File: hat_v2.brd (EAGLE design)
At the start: 65 x 56.5 mm, 18 parts, among them IC1 4N35

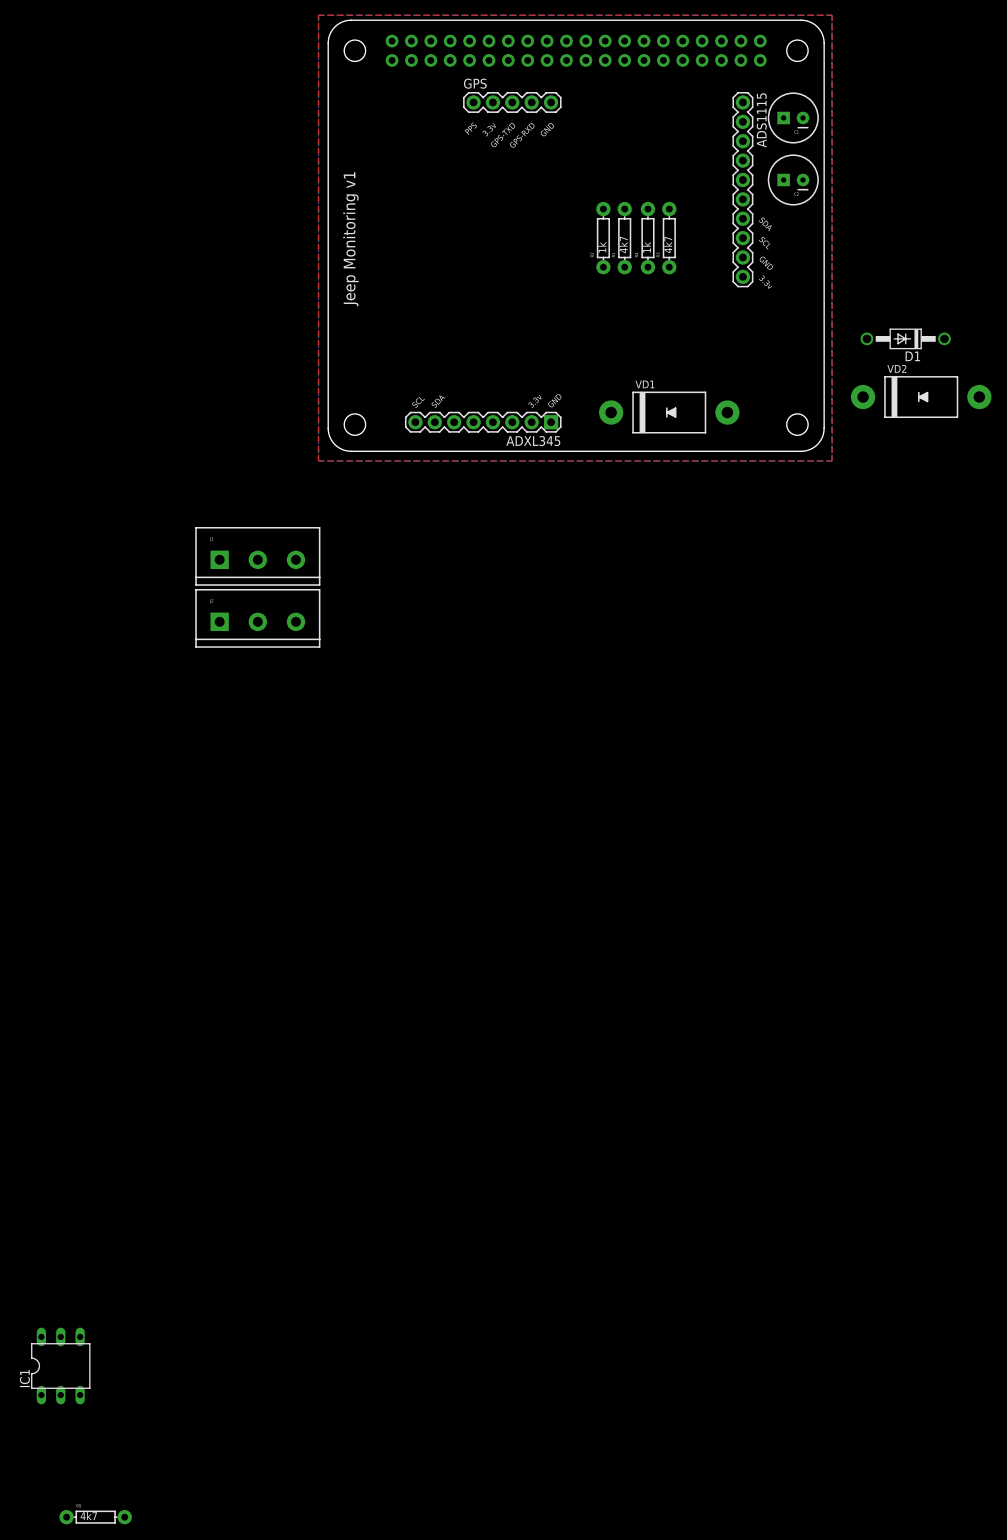
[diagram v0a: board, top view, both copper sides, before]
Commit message: V2 board done
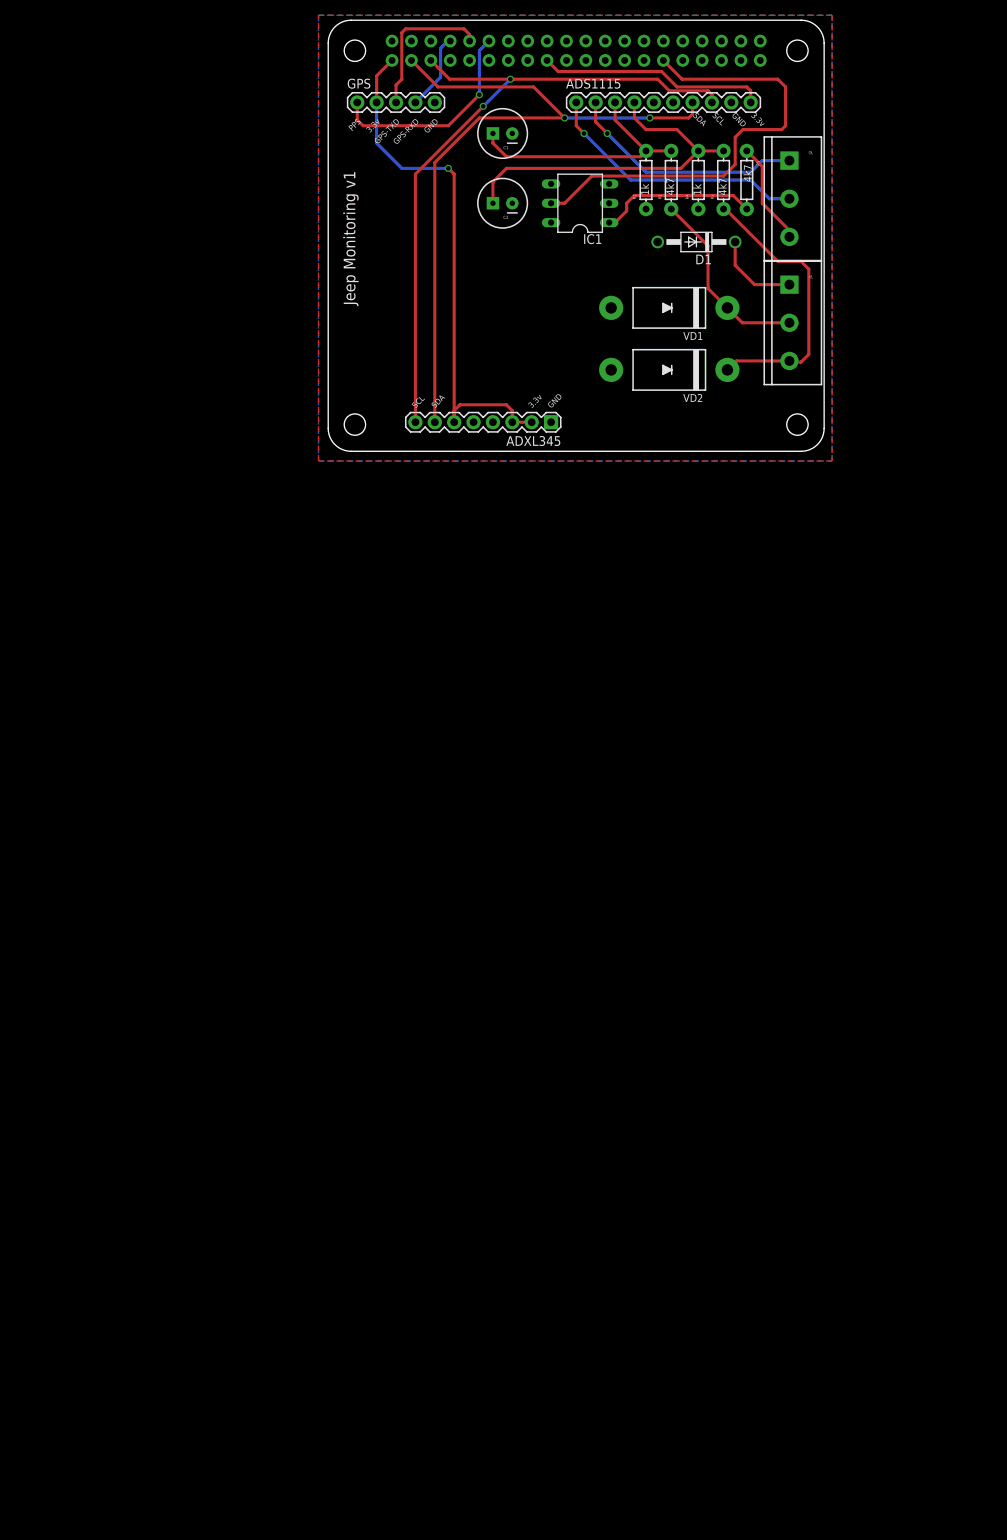
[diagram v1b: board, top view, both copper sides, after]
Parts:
- moved R5 194.9 mm to (54.9, 35.6), turned to 270 degrees
- moved IC1 166.9 mm to (33.0, 32.5), turned to 90 degrees
- moved J2 96.1 mm to (60.5, 38.1), turned to 270 degrees
- moved J1 82.9 mm to (60.5, 21.8), turned to 270 degrees
- moved C2 38.2 mm to (22.9, 32.5)
- moved C1 38.2 mm to (22.9, 41.7)
- moved VD2 33.2 mm to (44.7, 10.7), turned to 180 degrees
- moved D1 30.2 mm to (48.3, 27.4)
- moved ADS1115 21.8 mm to (32.5, 45.7), turned to 0 degrees
- moved GPS 15.2 mm to (3.81, 45.7)
- moved VD1 13.7 mm to (44.7, 18.8), turned to 180 degrees
- moved R3 10.4 mm to (51.8, 35.6)
- moved R4 10.1 mm to (48.5, 35.6)
- moved R1 9.76 mm to (45.0, 35.6)
- moved R2 9.45 mm to (41.7, 35.6)
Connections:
- net BAT-1: now also ADS1115.3; no longer ADS1115.4
- net BAT-2: now also ADS1115.4; no longer ADS1115.3
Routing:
- net 3.3V: track 0.00 -> 99.7 mm, vias 0 -> 1
- net SDA: track 0.00 -> 95.2 mm, vias 0 -> 2
- net SCL: track 0.00 -> 89.8 mm, vias 0 -> 2
- net GPIO5: track 0.00 -> 59.6 mm
- net BAT-2: track 0.00 -> 46.9 mm
- net BAT-2-INPUT: track 0.00 -> 37.3 mm
- net SHUNT-LOW-INPUT: track 0.00 -> 35.0 mm, vias 0 -> 1
- net BAT-1: track 0.00 -> 33.7 mm
- net SHUNT-HIGH-INPUT: track 0.00 -> 31.3 mm, vias 0 -> 1
- net GPIO18: track 0.00 -> 27.8 mm, vias 0 -> 1
- net BAT-1-INPUT: track 0.00 -> 24.9 mm
- net N$3: track 0.00 -> 20.8 mm
- net RXD: track 0.00 -> 19.7 mm
- net LINKED-INPUT: track 0.00 -> 13.6 mm
- net N$1: track 0.00 -> 11.2 mm
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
